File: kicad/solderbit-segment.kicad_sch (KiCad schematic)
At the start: 13 parts, among them J1 Conn_01x05_Pin, U1 PCF8574AT, U2 PCF8574N

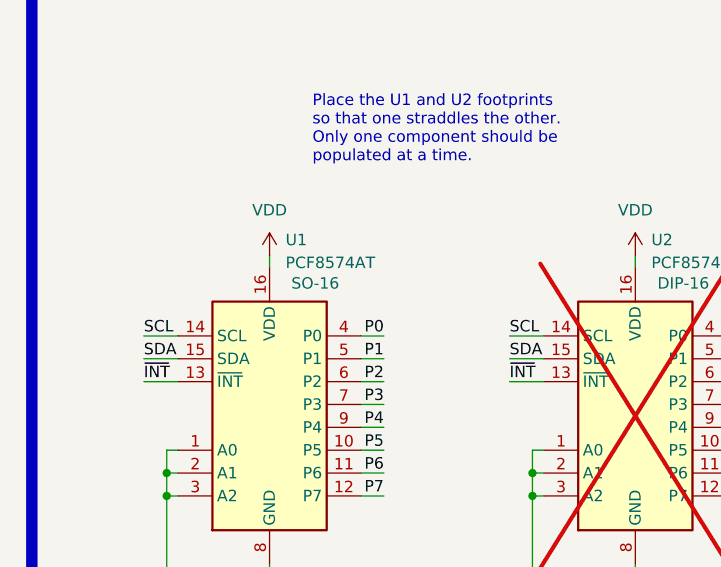
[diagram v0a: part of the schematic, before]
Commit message: Update documentation
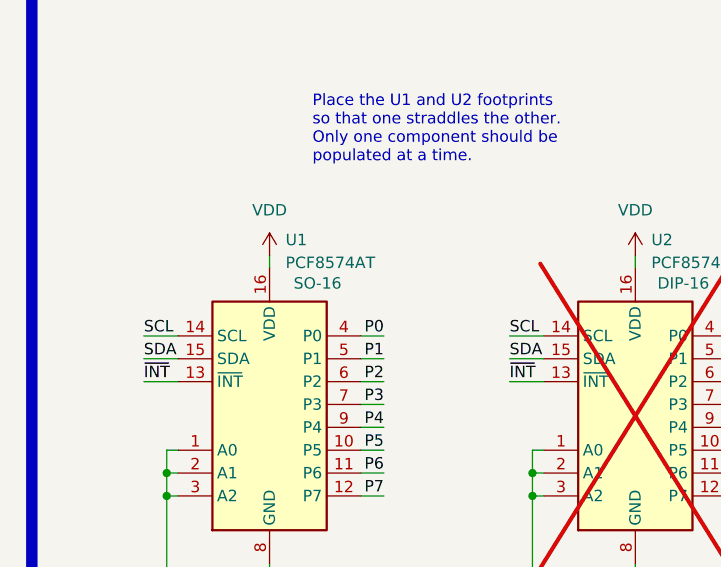
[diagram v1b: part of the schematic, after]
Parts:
- DS1: LCSC Part (none) -> C2913076; LCSC datasheet (none) -> https://www.lcsc.com/datasheet/C2913076.pdf; Onecall (none) -> 2682705; Onecall order code 2682705 -> (none); Package 10mm,SMD -> SMD; Type (none) -> Extended
- U1: Onecall (none) -> 2776146; Onecall order code 2776146 -> (none)
- U2: Onecall (none) -> 3124747; Onecall order code 3124747 -> (none)
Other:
- title: solder:bit Segment -> ${PROJECTNAME}
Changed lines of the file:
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@@
 	(paper "A4")
 	(title_block
-		(title "solder:bit Segment")
+		(title "${PROJECTNAME}")
 		(date "2026-02-16")
 		(rev "v0.1")
@@
 		)
 		(property "Package" "SO-16"
-			(at 50.8 58.928 0)
-			(effects
-				(font
-					(size 1.27 1.27)
-				)
-			)
-		)
-		(property "Onecall order code" "2776146"
-			(at 45.72 72.39 0)
-			(effects
-				(font
-					(size 1.27 1.27)
-				)
-				(hide yes)
-			)
-		)
-		(property "LCSC Part" ""
+			(at 51.054 58.928 0)
+			(effects
+				(font
+					(size 1.27 1.27)
+				)
+			)
+		)
+		(property "Onecall" "2776146"
 			(at 45.72 72.39 0)
 			(effects
@@
 			)
 		)
-		(property "Onecall order code" "3124747"
-			(at 86.36 72.39 0)
-			(effects
-				(font
-					(size 1.27 1.27)
-				)
-				(hide yes)
-			)
-		)
-		(property "LCSC Part" ""
+		(property "Onecall" "3124747"
 			(at 86.36 72.39 0)
 			(effects
@@
 			)
 		)
-		(property "Package" "10mm,SMD"
+		(property "Package" "SMD"
 			(at 180.34 34.544 0)
 			(effects
@@
 			)
 		)
-		(property "Onecall order code" "2682705"
+		(property "Onecall" "2682705"
 			(at 180.34 49.53 0)
 			(effects
@@
 			)
 		)
-		(property "LCSC Part" ""
+		(property "LCSC Part" "C2913076"
+			(at 180.34 49.53 0)
+			(effects
+				(font
+					(size 1.27 1.27)
+				)
+				(hide yes)
+			)
+		)
+		(property "Type" "Extended"
+			(at 180.34 49.53 0)
+			(effects
+				(font
+					(size 1.27 1.27)
+				)
+				(hide yes)
+			)
+		)
+		(property "LCSC datasheet" "https://www.lcsc.com/datasheet/C2913076.pdf"
 			(at 180.34 49.53 0)
 			(effects
@@
 			(at 180.34 109.22 0)
 			(effects
-				(font
-					(size 1.27 1.27)
-				)
-				(hide yes)
-			)
-		)
-		(property "LCSC Part" ""
-			(at 180.34 109.22 0)
-			(effects
